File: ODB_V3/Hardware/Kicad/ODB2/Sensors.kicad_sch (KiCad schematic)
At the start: 20 parts, among them U10 ADXL382-2BCCZ-RL7, U4 MS580301BA01-00, U6 BNO055, U9 MAX6612MXK

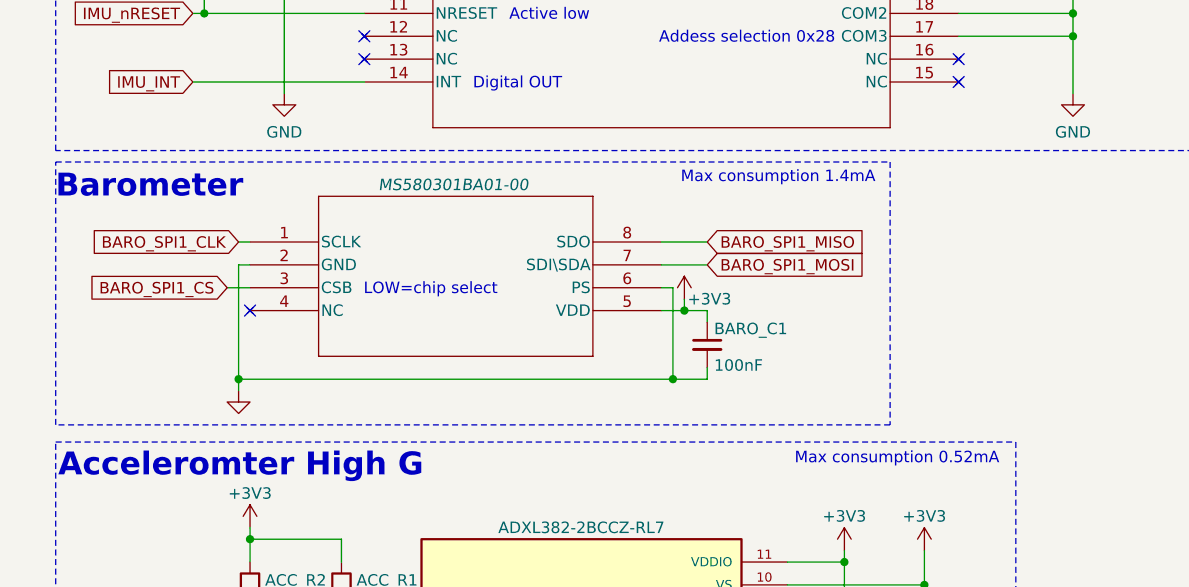
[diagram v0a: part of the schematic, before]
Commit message: wip: route qspi
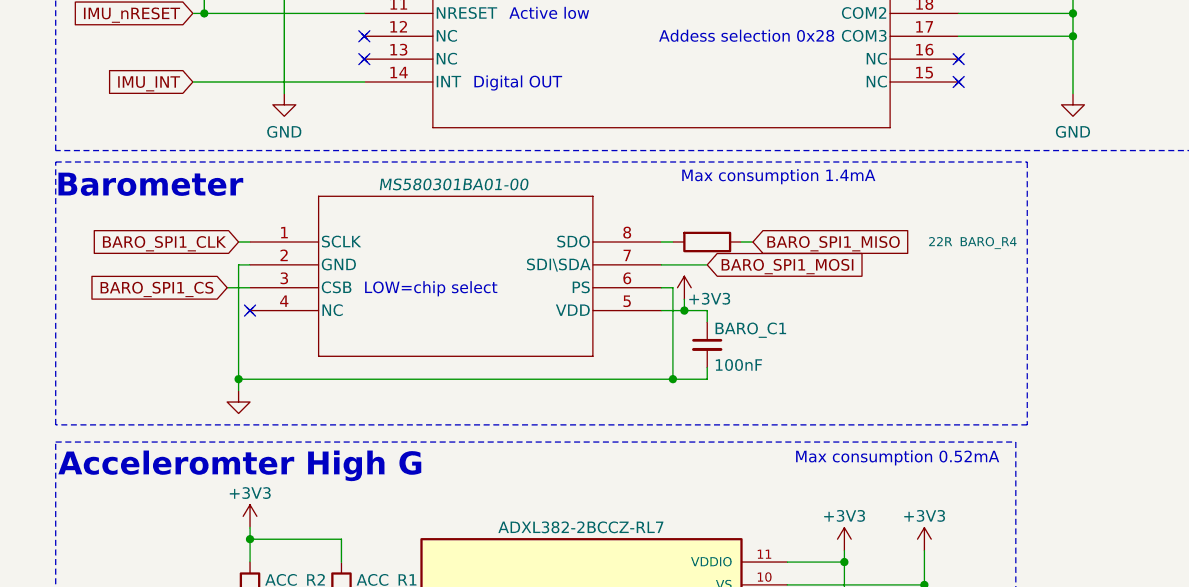
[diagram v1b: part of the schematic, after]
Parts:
- added BARO_R4: 22R, Resistor_SMD:R_0402_1005Metric, symbol Device:R
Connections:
- net BARO_SPI1_MISO: now also BARO_R4.1; no longer U4.8 (SDO)
- new net: BARO_R4.2, U4.8 (SDO)
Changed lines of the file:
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@@
 	(rectangle
 		(start 13.97 85.09)
-		(end 106.68 114.3)
+		(end 121.92 114.3)
 		(stroke
 			(width 0)
@@
 	(wire
 		(pts
+			(xy 90.17 93.98) (xy 91.44 93.98)
+		)
+		(stroke
+			(width 0)
+			(type default)
+		)
+	)
+	(wire
+		(pts
 			(xy 35.56 127) (xy 35.56 129.54)
 		)
@@
 	(wire
 		(pts
+			(xy 81.28 93.98) (xy 82.55 93.98)
+		)
+		(stroke
+			(width 0)
+			(type default)
+		)
+	)
+	(wire
+		(pts
 			(xy 99.06 157.48) (xy 99.06 160.02)
 		)
@@
 		(pts
 			(xy 110.49 160.02) (xy 101.6 160.02)
-		)
-		(stroke
-			(width 0)
-			(type default)
-		)
-	)
-	(wire
-		(pts
-			(xy 81.28 93.98) (xy 86.36 93.98)
 		)
 		(stroke
@@
 	(global_label "BARO_SPI1_MISO"
 		(shape input)
-		(at 86.36 93.98 0)
+		(at 91.44 93.98 0)
 		(fields_autoplaced yes)
 		(effects
@@
 		)
 		(property "Intersheetrefs" "${INTERSHEET_REFS}"
-			(at 105.1295 93.98 0)
+			(at 110.2095 93.98 0)
 			(effects
 				(font
@@
 					(unit 1)
 				)
+			)
+		)
+	)
+	(symbol
+		(lib_id "Device:R")
+		(at 86.36 93.98 270)
+		(unit 1)
+		(exclude_from_sim no)
+		(in_bom yes)
+		(on_board yes)
+		(dnp no)
+		(property "Reference" "BARO_R4"
+			(at 117.602 93.98 90)
+			(effects
+				(font
+					(size 1 1)
+				)
+			)
+		)
+		(property "Value" "22R"
+			(at 112.268 93.98 90)
+			(effects
+				(font
+					(size 1 1)
+				)
+			)
+		)
+		(property "Footprint" "Resistor_SMD:R_0402_1005Metric"
+			(at 86.36 92.202 90)
+			(effects
+				(font
+					(size 1 1)
+				)
+				(hide yes)
+			)
+		)
+		(property "Datasheet" "~"
+			(at 86.36 93.98 0)
+			(effects
+				(font
+					(size 1 1)
+				)
+				(hide yes)
+			)
+		)
+		(property "Description" ""
+			(at 86.36 93.98 0)
+			(effects
+				(font
+					(size 1.27 1.27)
+				)
+				(hide yes)
+			)
+		)
+		(pin "1"
+		)
+		(pin "2"
+		)
+		(instances
+			(project "ODB2"
+				(path "/4b06c5d1-aa8b-48ed-8972-b43a60cfab78/eac5f07f-d6a3-4c95-b286-7cebf46e30db"
+					(reference "BARO_R4")
+					(unit 1)
+				)
